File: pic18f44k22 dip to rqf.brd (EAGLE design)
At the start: 53.7 x 22.2 mm, 3 parts, among them IC1 PIC18F4455_TQFP

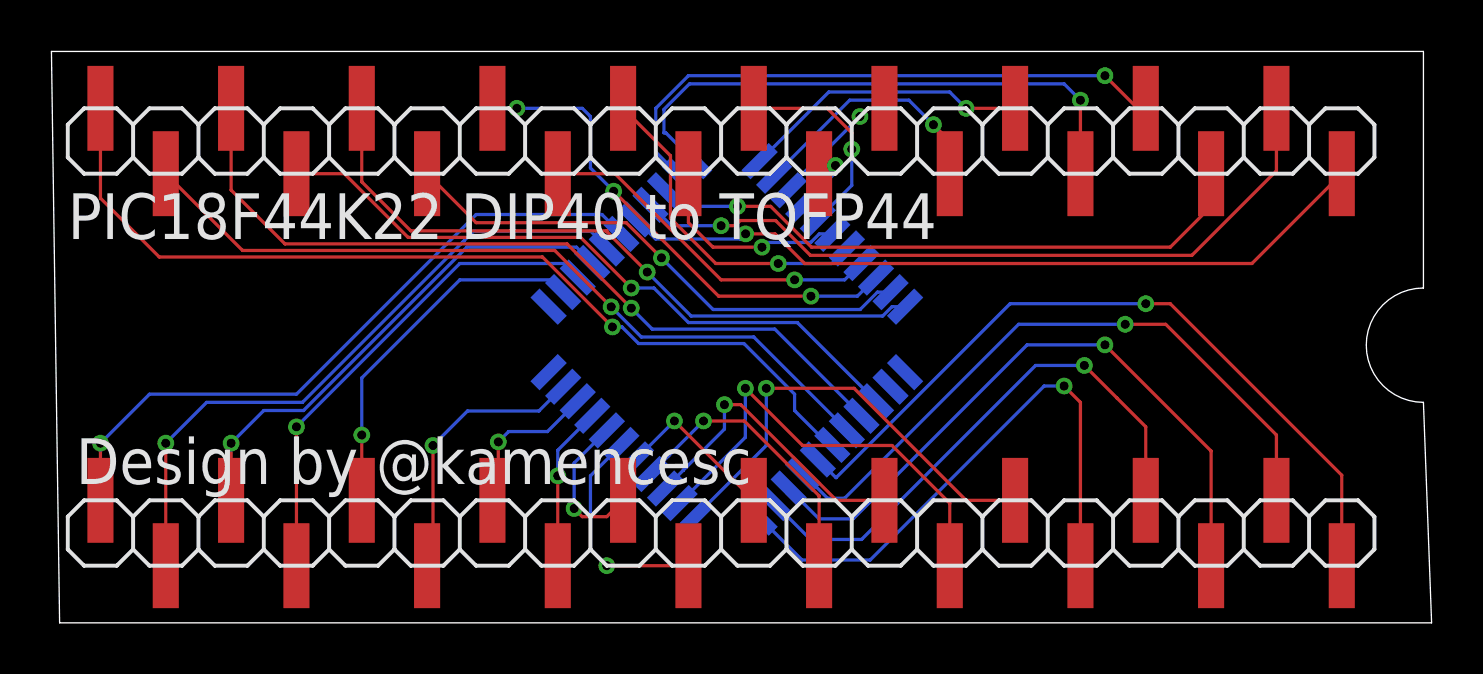
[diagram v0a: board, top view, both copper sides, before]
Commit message: Add files via upload
Adjustments...
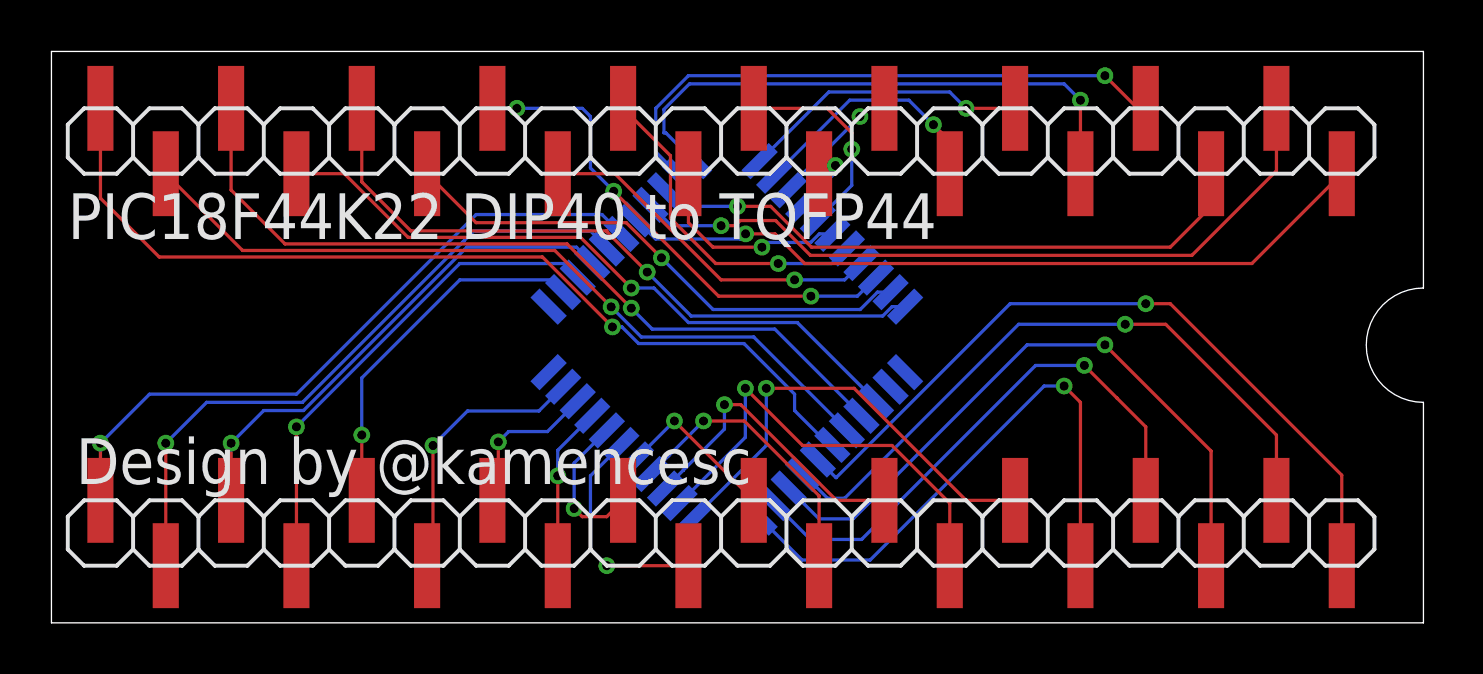
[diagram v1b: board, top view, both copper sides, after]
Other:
- board size 53.7 x 22.2 mm -> 53.3 x 22.2 mm
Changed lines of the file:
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@@
 <board>
 <plain>
-<wire x1="0.9525" y1="0.3175" x2="54.2925" y2="0.3175" width="0" layer="20"/>
+<wire x1="0.635" y1="0.3175" x2="53.975" y2="0.3175" width="0" layer="20"/>
 <wire x1="53.975" y1="22.5325" x2="0.635" y2="22.5325" width="0" layer="20"/>
-<wire x1="0.635" y1="22.5325" x2="0.9525" y2="0.3175" width="0" layer="20"/>
+<wire x1="0.635" y1="22.5325" x2="0.635" y2="0.3175" width="0" layer="20"/>
 <wire x1="52.705" y1="21.9075" x2="52.705" y2="13.6525" width="0.1524" layer="22"/>
 <wire x1="52.705" y1="8.5725" x2="52.705" y2="0.9525" width="0.1524" layer="22"/>
@@
 <wire x1="53.975" y1="13.335" x2="53.975" y2="8.89" width="0" layer="20" curve="180"/>
 <wire x1="53.975" y1="13.335" x2="53.975" y2="22.5325" width="0" layer="20"/>
-<wire x1="53.975" y1="8.89" x2="54.2925" y2="0.3175" width="0" layer="20"/>
+<wire x1="53.975" y1="8.89" x2="53.975" y2="0.3175" width="0" layer="20"/>
 <text x="1.27" y="15.24" size="1.778" layer="25">PIC18F44K22 DIP40 to TQFP44</text>
 <text x="1.5875" y="5.715" size="1.778" layer="25">Design by @kamencesc</text>
